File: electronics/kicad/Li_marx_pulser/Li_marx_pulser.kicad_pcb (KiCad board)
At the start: 2 copper layers, 61 parts, among them Q1 MMBT5551, Q10 MMBT5551, Q11 MMBT5551, Q12 MMBT5551, Q13 MMBT5551, Q14 MMBT5551, Q15 MMBT5551, Q2 MMBT5551, Q3 MMBT5551, Q4 MMBT5551, Q5 MMBT5551, Q6 MMBT5551, Q7 MMBT5551, Q8 MMBT5551, Q9 MMBT5551

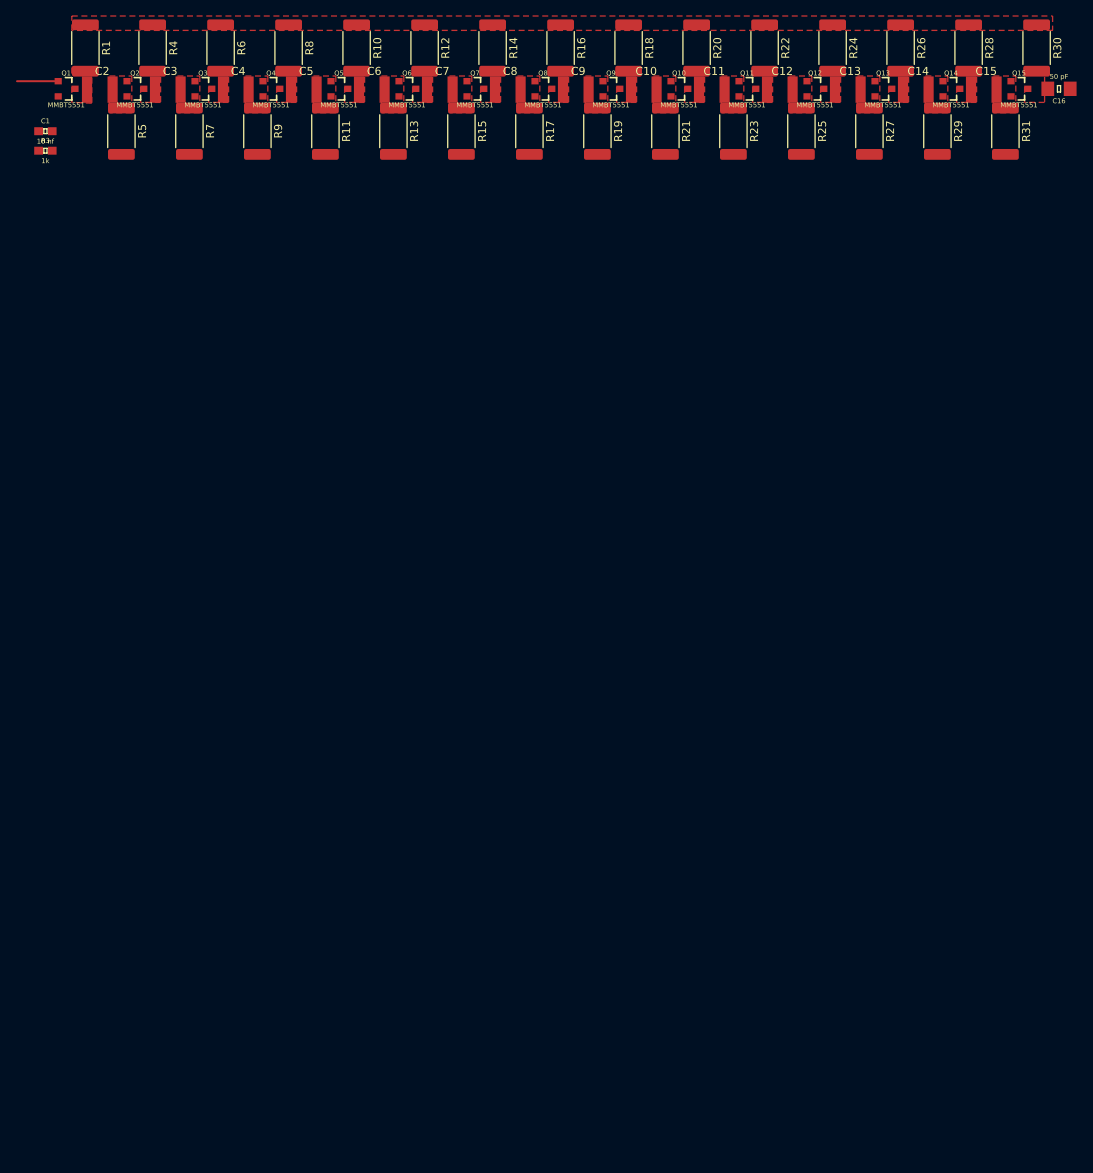
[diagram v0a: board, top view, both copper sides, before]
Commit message: Progress
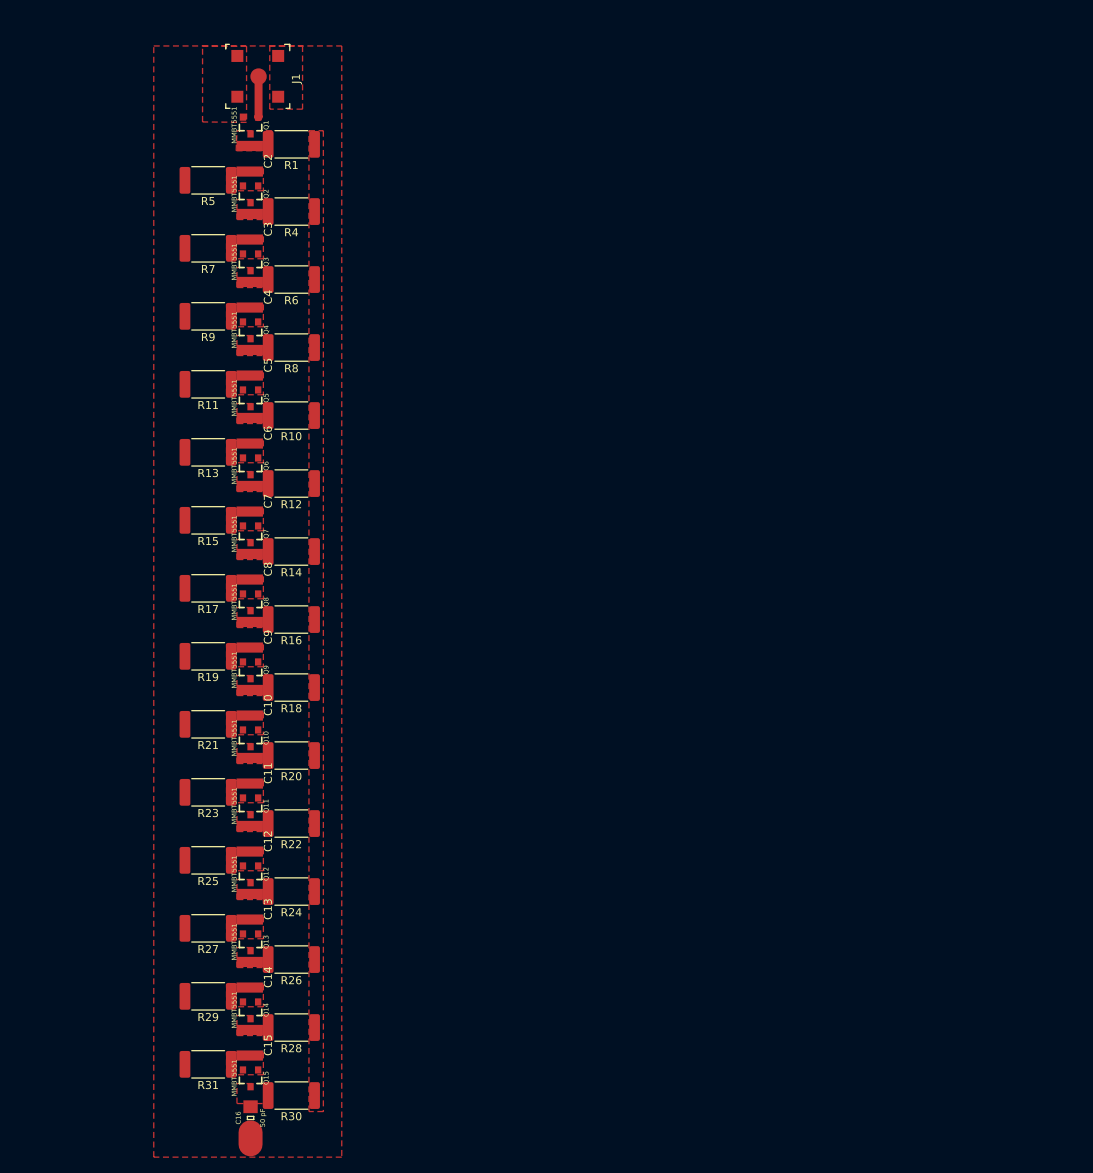
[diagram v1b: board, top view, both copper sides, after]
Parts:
- removed C1: 10 nf, Capacitors:0603
- removed R3: 1k, Capacitors:0603
- added J1: CONSMA001-SMD-G, digikey-footprints:RF_SMA_Receptical_Vertical_CONSMA001-SMD-G, F.Cu at (42.8, 62.0)
- moved C16 163.6 mm to (41.9, 192.2), turned to 90 degrees
- moved R30 160.7 mm to (47.0, 189.4), turned to 180 degrees
- moved Q15 156.6 mm to (41.9, 187.2), turned to 180 degrees
- moved R31 153.4 mm to (36.6, 185.5), turned to 180 degrees
- moved C15 151.1 mm to (45.2, 182.8), turned to 270 degrees
- moved R28 148.9 mm to (47.0, 180.9), turned to 180 degrees
- moved Q14 144.7 mm to (41.9, 178.7), turned to 180 degrees
- moved R29 141.4 mm to (36.6, 177.0), turned to 180 degrees
- moved C14 139.2 mm to (45.2, 174.3), turned to 270 degrees
- moved R26 137.0 mm to (47.0, 172.4), turned to 180 degrees
- moved Q13 132.7 mm to (41.9, 170.2), turned to 180 degrees
- moved R27 129.5 mm to (36.6, 168.5), turned to 180 degrees
- moved C13 127.4 mm to (45.2, 165.8), turned to 270 degrees
- moved R24 125.3 mm to (47.0, 163.9), turned to 180 degrees
- moved Q12 120.9 mm to (41.9, 161.7), turned to 180 degrees
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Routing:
- net Net-(C16-Pad1): track 0.00 -> 1.50 mm
- added copper zone on F.Cu, net GND
